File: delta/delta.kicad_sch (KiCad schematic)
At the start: 12 parts, among them U1 ATtiny1616-M

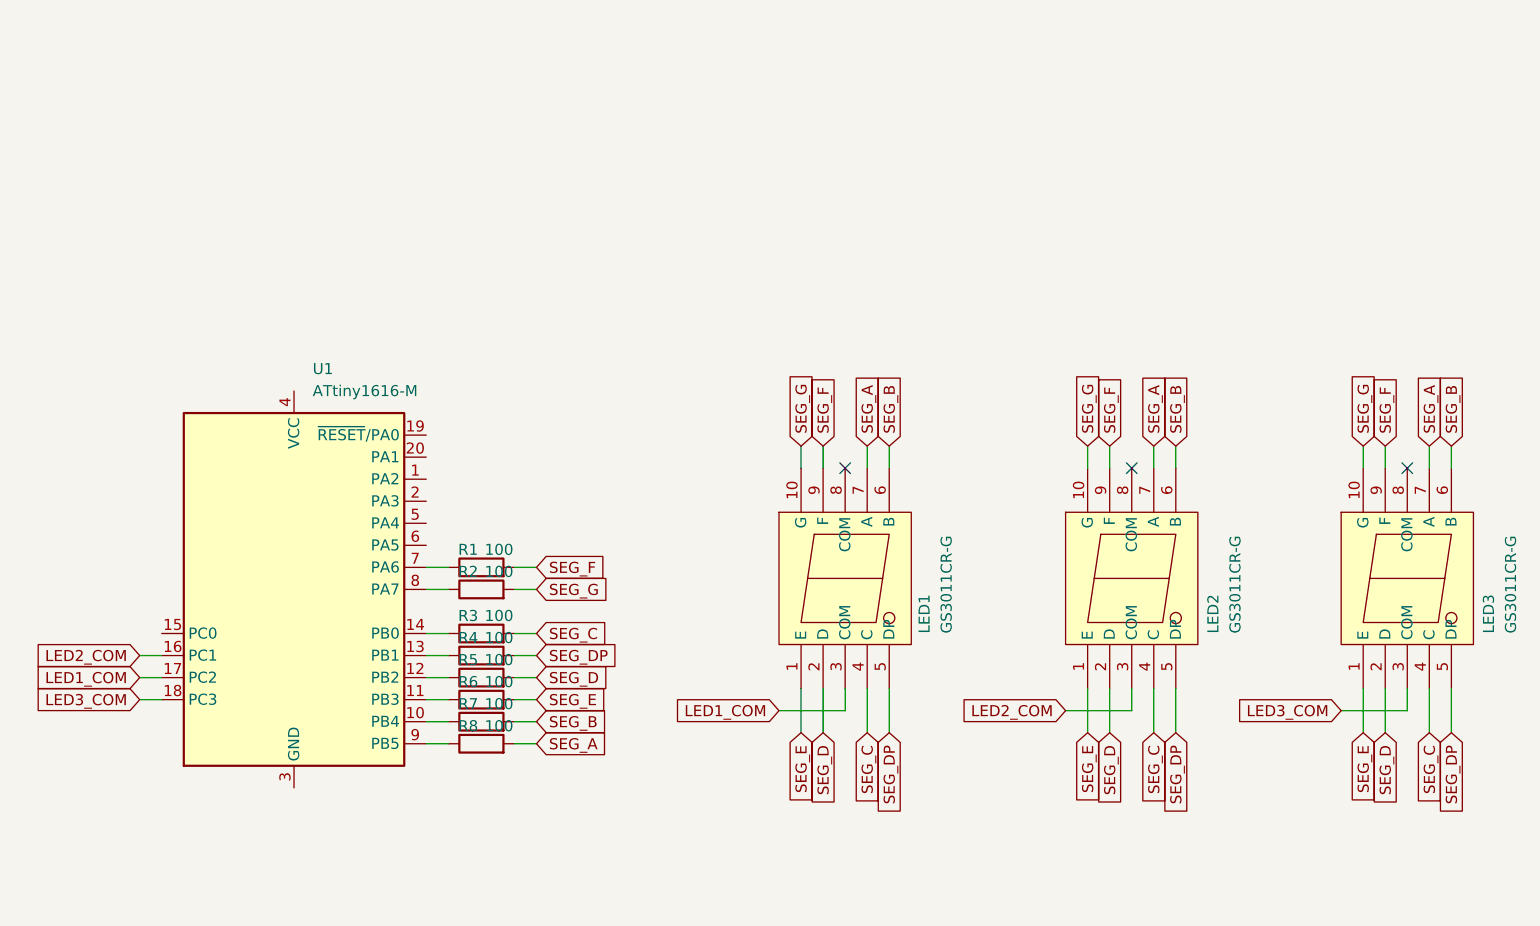
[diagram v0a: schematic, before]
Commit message: yes
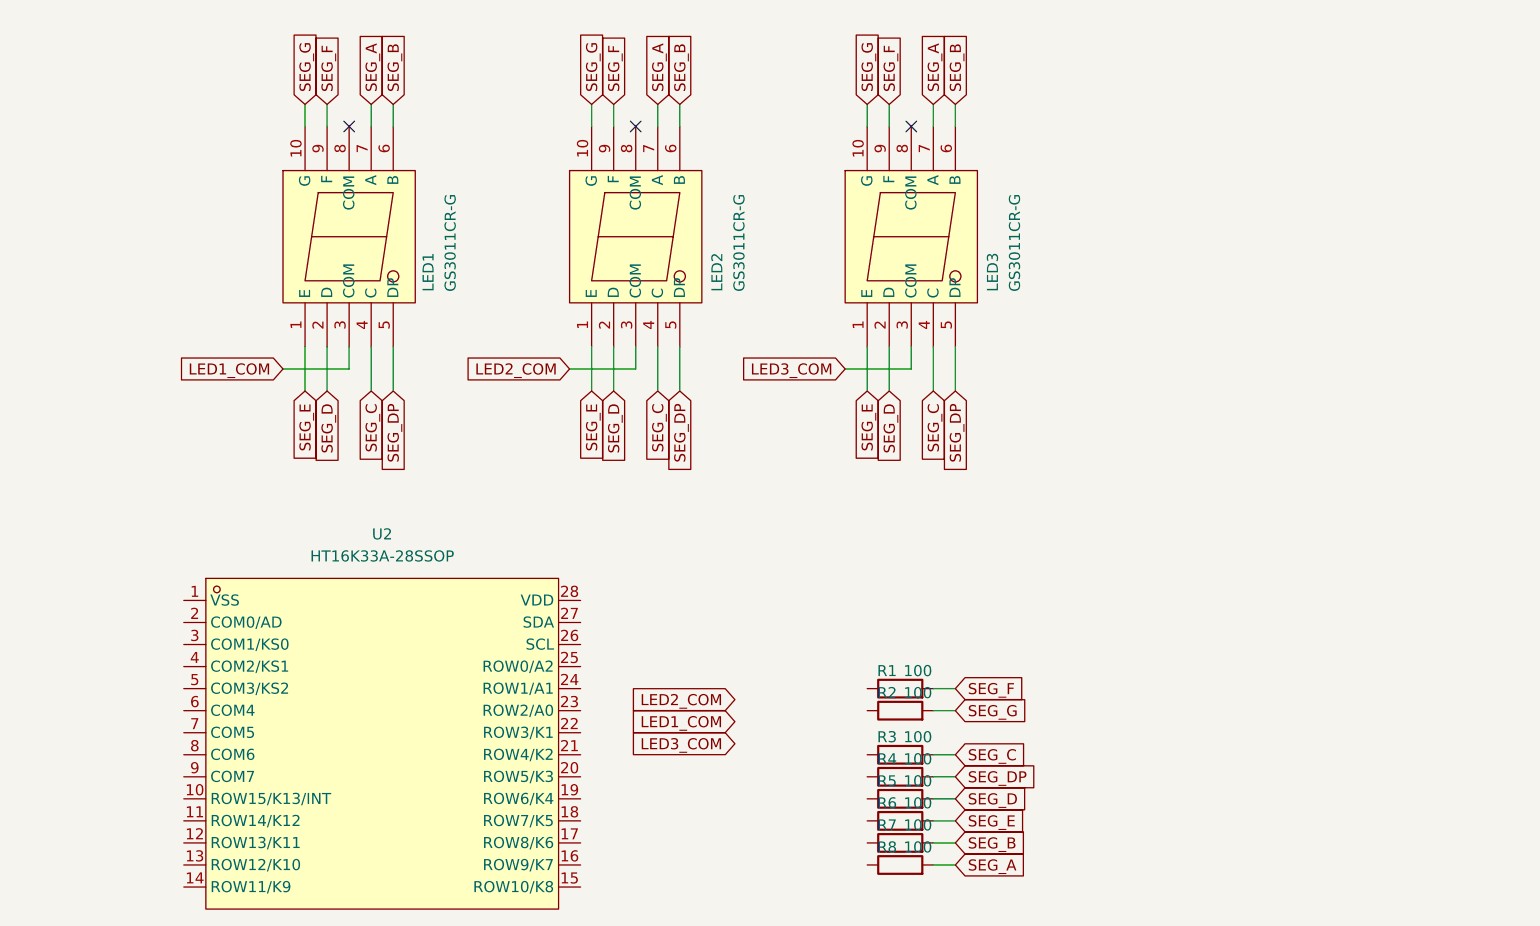
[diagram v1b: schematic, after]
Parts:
- removed U1: ATtiny1616-M, Package_DFN_QFN:VQFN-20-1EP_3x3mm_P0.4mm_EP1.7x1.7mm, symbol MCU_Microchip_ATtiny:ATtiny1616-M
- added U2: HT16K33A-28SSOP, easyeda2kicad:SSOP-28_L9.9-W3.9-P0.64-LS6.0-BL, symbol easyeda2kicad:HT16K33A-28SSOP
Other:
- moved on the sheet: LED1, LED2, LED3
